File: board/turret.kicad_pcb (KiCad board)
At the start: 2 copper layers, 54 parts, among them M1 SRV_LAS, M2 SRV_SEN, Q1 BC848, SW1 SW_Push, U1 STM32F103CBTx, U2 W25Q16JLSSIG, U3 TPA2005D1DGN, U4 TPS61322xADBV, U5 TLV70028_SOT23-5

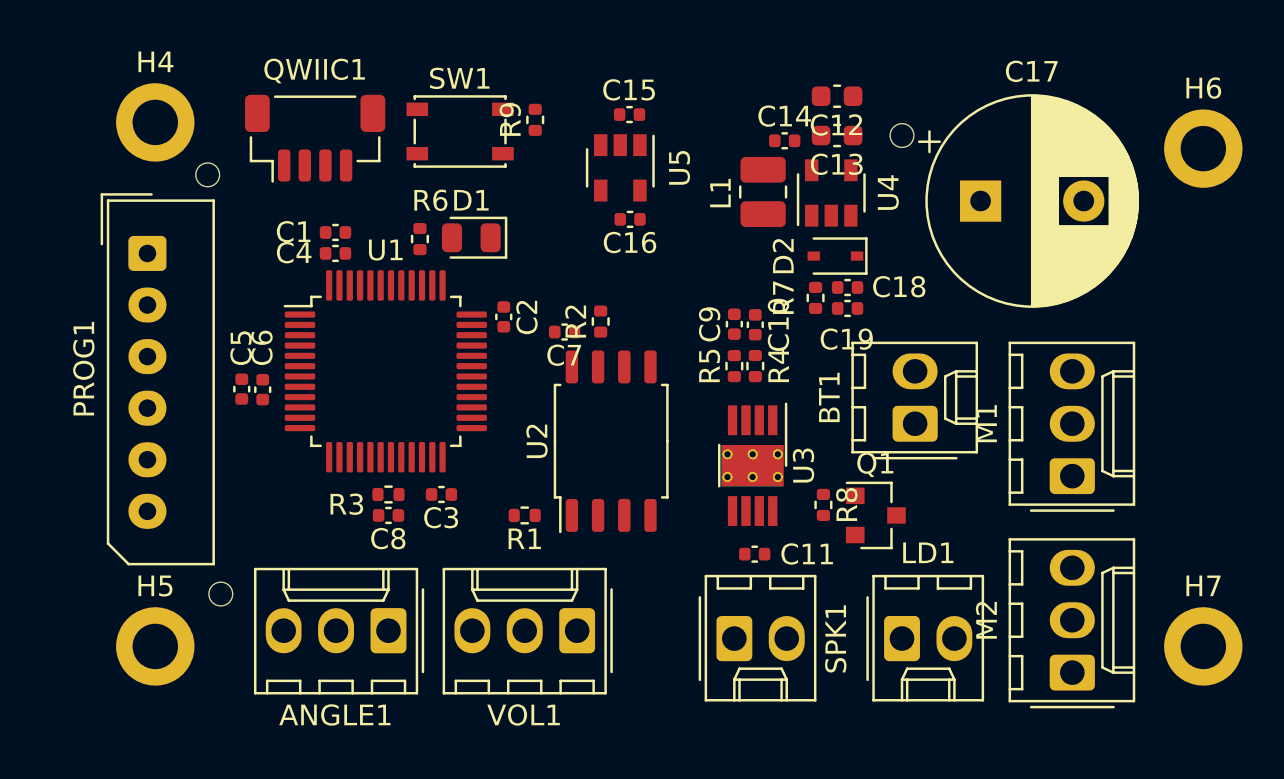
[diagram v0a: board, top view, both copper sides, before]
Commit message: Board layout complete
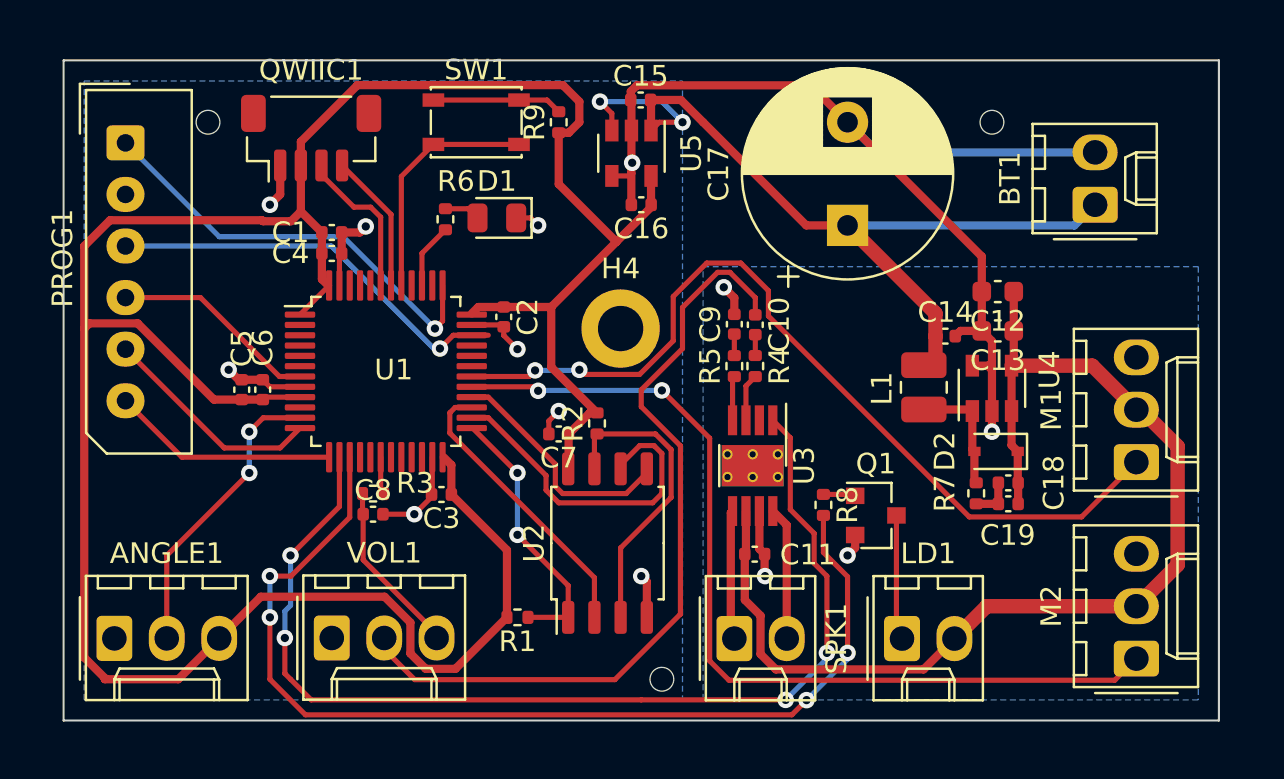
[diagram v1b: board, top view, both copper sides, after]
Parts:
- removed H5, H6, H7: MountingHole_Pad, MountingHole:MountingHole_2.2mm_M2_DIN965_Pad
- moved H4 24.7 mm to (154.0, 90.0)
- moved H2 21.8 mm to (156.0, 107.0)
- moved BT1 13.7 mm to (177.0, 84.0)
- moved ANGLE1 13.3 mm to (129.5, 105.0), turned to 0 degrees
- moved C12 12.3 mm to (172.3, 88.2)
- moved C13 12.3 mm to (172.3, 90.1)
- moved L1 12.3 mm to (168.7, 92.8)
- moved C14 12.3 mm to (169.7, 90.4)
- moved C18 12.3 mm to (172.8, 97.5)
- moved C19 12.3 mm to (172.8, 98.5)
- moved D2 12.3 mm to (172.2, 96.0)
- moved R7 12.3 mm to (171.2, 98.0)
- moved U4 12.3 mm to (172.0, 92.9)
- moved VOL1 11.9 mm to (140.0, 105.0), turned to 0 degrees
- moved C17 6.56 mm to (165.0, 85.0), turned to 90 degrees
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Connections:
- H4 pad 1: GND -> GNDA
- U1 pad 10: (no net) -> unconnected-(U1-Pad10)
- U1 pad 16: (no net) -> unconnected-(U1-Pad16)
- U1 pad 17: (no net) -> unconnected-(U1-Pad17)
- U1 pad 19: (no net) -> unconnected-(U1-Pad19)
- U1 pad 2: (no net) -> unconnected-(U1-Pad2)
- U1 pad 20: (no net) -> unconnected-(U1-Pad20)
- U1 pad 21: (no net) -> unconnected-(U1-Pad21)
- U1 pad 22: (no net) -> unconnected-(U1-Pad22)
- U1 pad 3: (no net) -> unconnected-(U1-Pad3)
- U1 pad 31: (no net) -> unconnected-(U1-Pad31)
- U1 pad 32: (no net) -> unconnected-(U1-Pad32)
- U1 pad 33: (no net) -> unconnected-(U1-Pad33)
- U1 pad 38: (no net) -> unconnected-(U1-Pad38)
- U1 pad 4: (no net) -> unconnected-(U1-Pad4)
- U1 pad 40: (no net) -> unconnected-(U1-Pad40)
- U1 pad 44: (no net) -> unconnected-(U1-Pad44)
- U1 pad 45: (no net) -> unconnected-(U1-Pad45)
- U1 pad 46: (no net) -> unconnected-(U1-Pad46)
- U1 pad 5: (no net) -> unconnected-(U1-Pad5)
- U1 pad 6: (no net) -> unconnected-(U1-Pad6)
- U3 pad 2: (no net) -> unconnected-(U3-Pad2)
- U3 pad 9: (no net) -> GNDA
- U4 pad 3: (no net) -> +5V
- U4 pad 5: (no net) -> GNDA
- U5 pad 4: (no net) -> GNDA
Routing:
- net VDD: track 0.00 -> 133.4 mm
- net GNDA: track 0.00 -> 78.8 mm, vias 0 -> 13
- net +5V: track 0.00 -> 55.8 mm
- net /AU_ENAB: track 0.00 -> 51.9 mm, vias 0 -> 4
- net /LASER: track 0.00 -> 50.2 mm, vias 0 -> 4
- net /SRV_SEN: track 0.00 -> 44.9 mm, vias 0 -> 2
- net /SRV_LAS: track 0.00 -> 42.9 mm, vias 0 -> 2
- net Net-(BT1-Pad1): track 0.00 -> 42.5 mm, vias 0 -> 2
- net Net-(C10-Pad1): track 0.00 -> 38.9 mm
- net /SWCLK: track 0.00 -> 21.0 mm, vias 0 -> 1
- net /SWDIO: track 0.00 -> 19.9 mm, vias 0 -> 1
- net /SPI_SCK: track 0.00 -> 16.2 mm
- net Net-(R2-Pad1): track 0.00 -> 14.8 mm
- net /ANGLE_POT: track 0.00 -> 14.4 mm, vias 0 -> 2
- net /SPI_MISO: track 0.00 -> 14.0 mm
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- added copper zone on B.Cu, net GNDA
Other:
- board outline added: 56 x 32 mm
